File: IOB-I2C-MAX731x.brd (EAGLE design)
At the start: 71.1 x 33 mm, 9 parts, among them IC1 MAX7311, SW1 A0, SW2 A1, SW3 A2

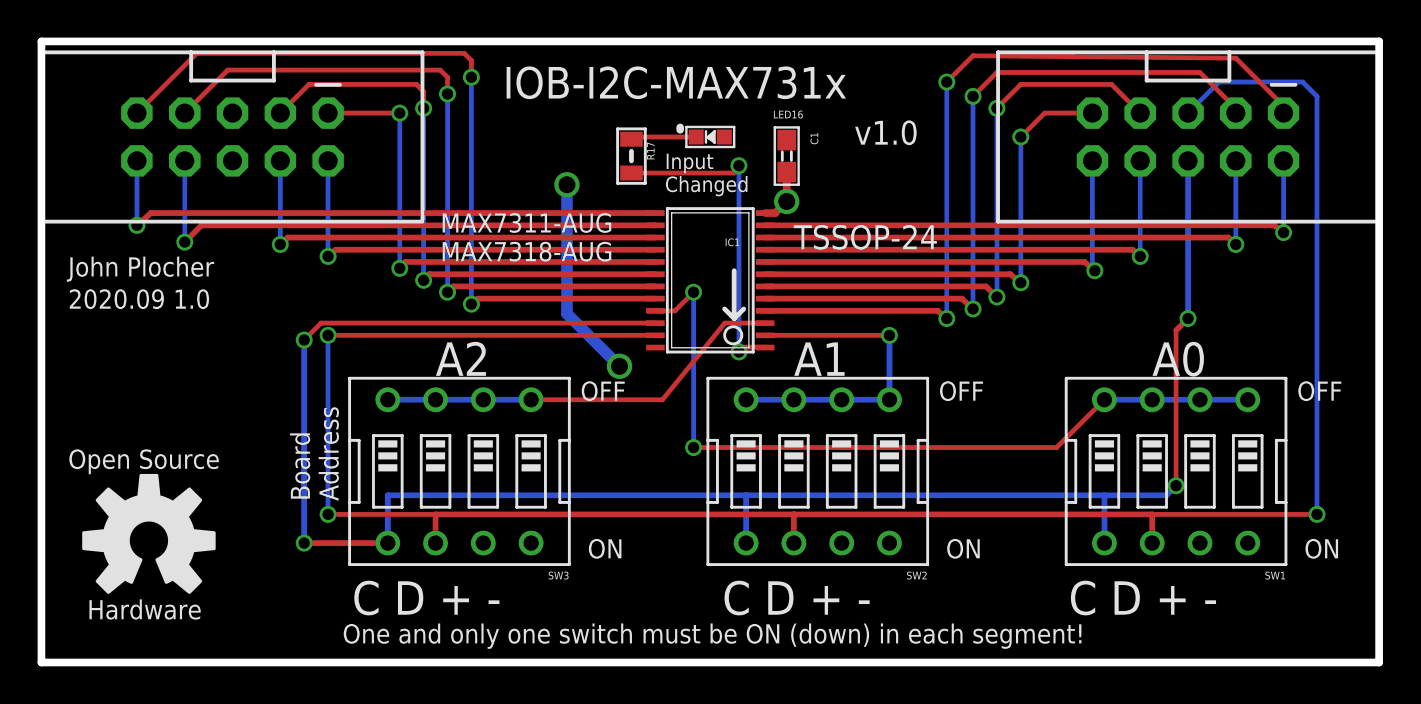
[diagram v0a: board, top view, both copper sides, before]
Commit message: cleanup layout
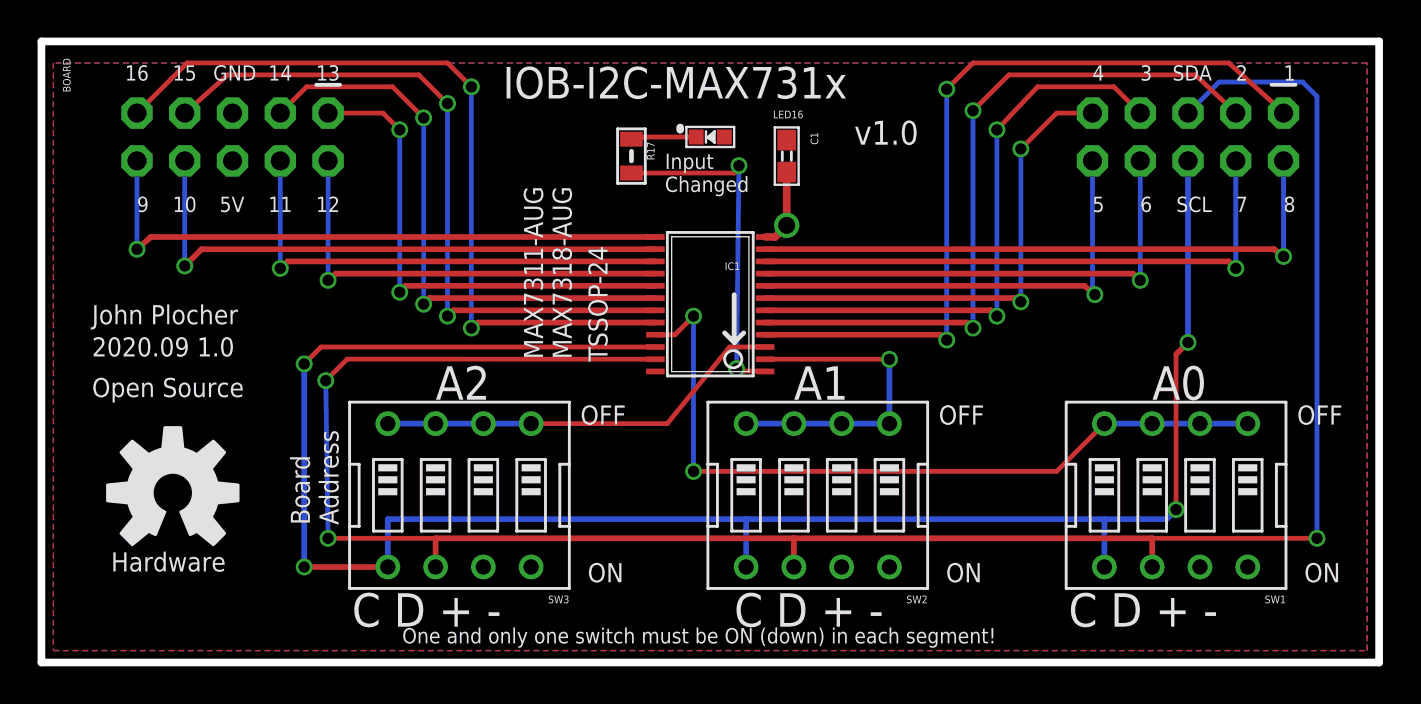
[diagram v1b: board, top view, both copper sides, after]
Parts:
- BOARD: value I2C-EXPANDER -> CONNECTOR-I2C-EXPANDER
- moved U$1 2.84 mm to (6.99, 9.02)
- moved IC1 1.27 mm to (35.6, 19.1)
- moved SW1 1.27 mm to (60.3, 8.89)
- moved SW2 1.27 mm to (41.3, 8.89)
- moved SW3 1.27 mm to (22.2, 8.89)
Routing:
- net VCC: track 10.8 -> 0.00 mm, vias 2 -> 0
- net P11: track 24.5 -> 25.8 mm
- net P7: track 29.6 -> 30.9 mm
- net P9: track 31.2 -> 32.5 mm
- net P6: track 25.2 -> 26.4 mm
- net P12: track 22.6 -> 23.9 mm
- net P10: track 29.7 -> 31.0 mm
- net GND: track 2.96 -> 4.23 mm
- net SCL: track 101.6 -> 102.9 mm
- net P8: track 31.5 -> 32.8 mm
- net P5: track 23.7 -> 24.9 mm
- net !INT: track 17.4 -> 18.3 mm
- net P13: track 25.8 -> 26.6 mm
- net SDA: track 114.2 -> 114.9 mm
- net P4: track 25.8 -> 26.4 mm
